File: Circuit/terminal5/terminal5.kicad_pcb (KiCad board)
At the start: 2 copper layers, 14 parts, among them J1 Conn_01x05_Male, J2 Conn_02x08_Odd_Even, J3 Conn_01x02_Male, U1 4051

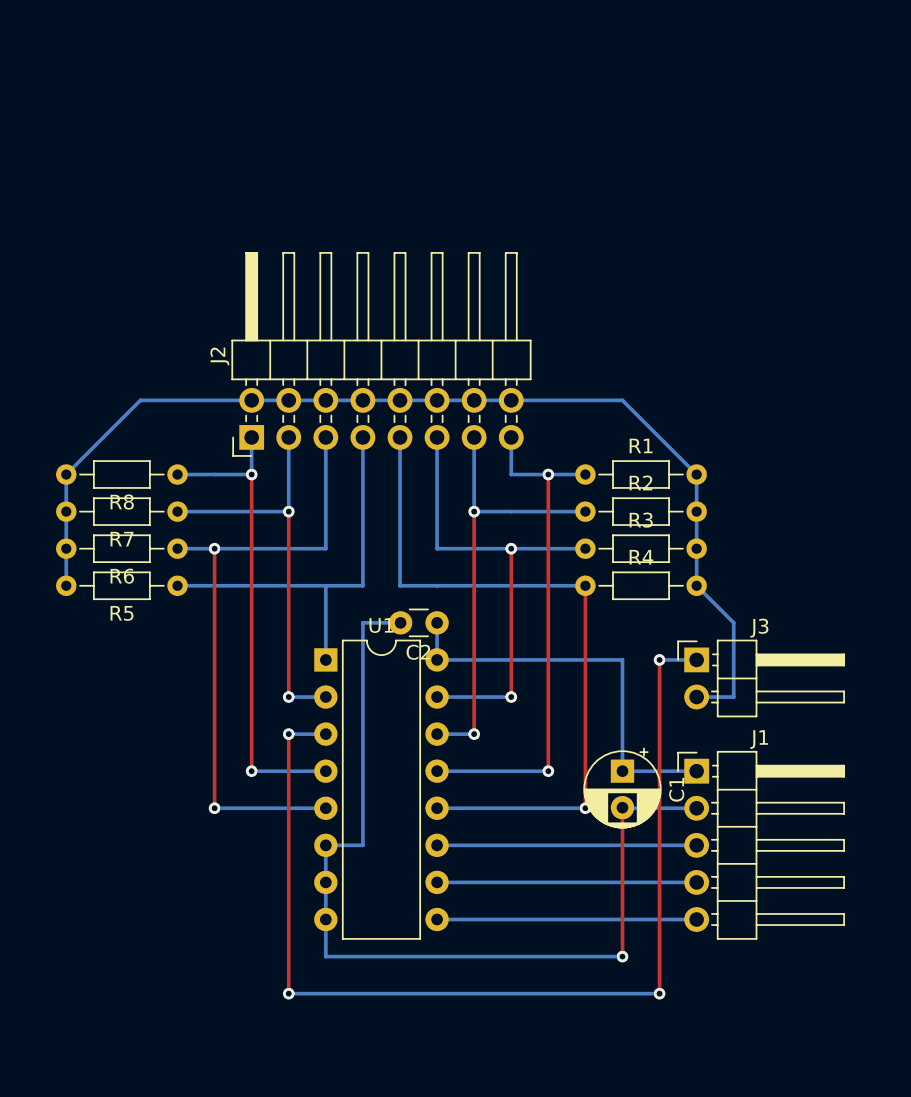
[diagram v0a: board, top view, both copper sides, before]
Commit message: ECM対策
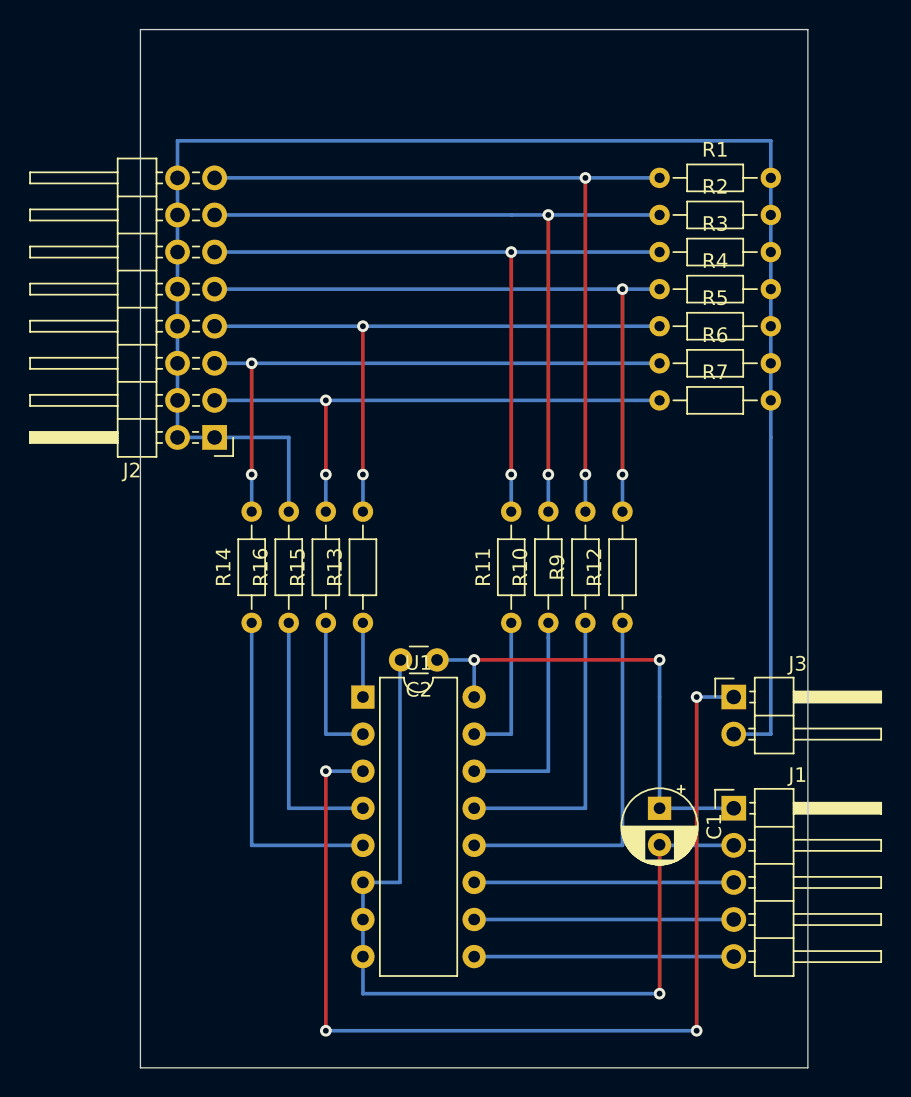
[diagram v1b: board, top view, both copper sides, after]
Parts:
- removed R8: 10k, Resistor_THT:R_Axial_DIN0204_L3.6mm_D1.6mm_P7.62mm_Horizontal
- added R10: 220, Resistor_THT:R_Axial_DIN0204_L3.6mm_D1.6mm_P7.62mm_Horizontal, F.Cu at (132.1, 73.7)
- added R11: 220, Resistor_THT:R_Axial_DIN0204_L3.6mm_D1.6mm_P7.62mm_Horizontal, F.Cu at (129.5, 73.7)
- added R12: 220, Resistor_THT:R_Axial_DIN0204_L3.6mm_D1.6mm_P7.62mm_Horizontal, F.Cu at (137.2, 73.7)
- added R13: 220, Resistor_THT:R_Axial_DIN0204_L3.6mm_D1.6mm_P7.62mm_Horizontal, F.Cu at (119.4, 73.7)
- added R14: 220, Resistor_THT:R_Axial_DIN0204_L3.6mm_D1.6mm_P7.62mm_Horizontal, F.Cu at (111.8, 73.7)
- added R15: 220, Resistor_THT:R_Axial_DIN0204_L3.6mm_D1.6mm_P7.62mm_Horizontal, F.Cu at (116.8, 73.7)
- added R16: 220, Resistor_THT:R_Axial_DIN0204_L3.6mm_D1.6mm_P7.62mm_Horizontal, F.Cu at (114.3, 73.7)
- added R9: 220, Resistor_THT:R_Axial_DIN0204_L3.6mm_D1.6mm_P7.62mm_Horizontal, F.Cu at (134.6, 73.7)
- moved R5 37.5 mm to (139.7, 53.3), turned to 0 degrees
- moved R6 35.4 mm to (139.7, 55.9), turned to 0 degrees
- moved R7 33.9 mm to (139.7, 58.4), turned to 0 degrees
- moved R2 20.9 mm to (139.7, 45.7)
- moved R4 20.9 mm to (139.7, 50.8)
- moved R1 20.9 mm to (139.7, 43.2)
- moved R3 20.9 mm to (139.7, 48.3)
- moved C1 3.59 mm to (139.7, 86.4)
- moved J1 3.59 mm to (144.8, 86.4)
- moved J3 3.59 mm to (144.8, 78.7)
- moved U1 3.59 mm to (119.4, 78.7)
- moved C2 2.54 mm to (124.5, 76.2)
- moved J2 2.54 mm to (109.2, 61.0), turned to 180 degrees
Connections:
- J2 pad 10: Net-(J2-Pad10) -> Net-(J2-Pad1)
- J2 pad 12: Net-(J2-Pad10) -> Net-(J2-Pad1)
- J2 pad 14: Net-(J2-Pad10) -> Net-(J2-Pad1)
- J2 pad 16: Net-(J2-Pad10) -> Net-(J2-Pad1)
- J2 pad 2: Net-(J2-Pad10) -> Net-(J2-Pad1)
- J2 pad 4: Net-(J2-Pad10) -> Net-(J2-Pad1)
- J2 pad 6: Net-(J2-Pad10) -> Net-(J2-Pad1)
- J2 pad 8: Net-(J2-Pad10) -> Net-(J2-Pad1)
- J3 pad 2: Net-(J2-Pad10) -> Net-(J2-Pad1)
- R1 pad 2: Net-(J2-Pad10) -> Net-(J2-Pad1)
- R2 pad 2: Net-(J2-Pad10) -> Net-(J2-Pad1)
- R3 pad 2: Net-(J2-Pad10) -> Net-(J2-Pad1)
- R4 pad 2: Net-(J2-Pad10) -> Net-(J2-Pad1)
- R5 pad 2: Net-(J2-Pad10) -> Net-(J2-Pad1)
- R6 pad 2: Net-(J2-Pad10) -> Net-(J2-Pad1)
- R7 pad 2: Net-(J2-Pad10) -> Net-(J2-Pad1)
- U1 pad 1: Net-(J2-Pad7) -> Net-(R13-Pad1)
- U1 pad 12: Net-(J2-Pad9) -> Net-(R12-Pad1)
- U1 pad 13: Net-(J2-Pad15) -> Net-(R9-Pad1)
- U1 pad 14: Net-(J2-Pad13) -> Net-(R10-Pad1)
- U1 pad 15: Net-(J2-Pad11) -> Net-(R11-Pad1)
- U1 pad 2: Net-(J2-Pad3) -> Net-(R15-Pad1)
- U1 pad 4: Net-(J2-Pad1) -> Net-(R16-Pad1)
- U1 pad 5: Net-(J2-Pad5) -> Net-(R14-Pad1)
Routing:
- net Net-(J2-Pad1): track 33.0 -> 116.8 mm, vias 2 -> 0
- net Net-(J2-Pad10): track 73.8 -> 0.00 mm
- net Net-(R12-Pad1): track 0.00 -> 25.4 mm
- net Net-(R14-Pad1): track 0.00 -> 22.9 mm
- net Net-(R9-Pad1): track 0.00 -> 20.3 mm
- net Net-(J2-Pad13): track 30.5 -> 50.8 mm
- net Net-(R16-Pad1): track 0.00 -> 17.8 mm
- net Net-(J2-Pad15): track 35.6 -> 53.3 mm
- net Net-(R10-Pad1): track 0.00 -> 15.2 mm
- net Net-(J2-Pad7): track 27.9 -> 43.2 mm, vias 0 -> 2
- net Net-(J2-Pad11): track 33.0 -> 48.3 mm
- net Net-(J2-Pad3): track 27.9 -> 38.1 mm
- net Net-(R15-Pad1): track 0.00 -> 10.2 mm
- net Net-(R11-Pad1): track 0.00 -> 10.2 mm
- net Net-(R13-Pad1): track 0.00 -> 5.08 mm
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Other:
- board outline added: 45.7 x 71.1 mm
- board text added: "Akizuki Type C Board (17x27)"
